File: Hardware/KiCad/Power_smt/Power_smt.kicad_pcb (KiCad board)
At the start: 2 copper layers, 38.1 x 25.4 mm, 11 parts

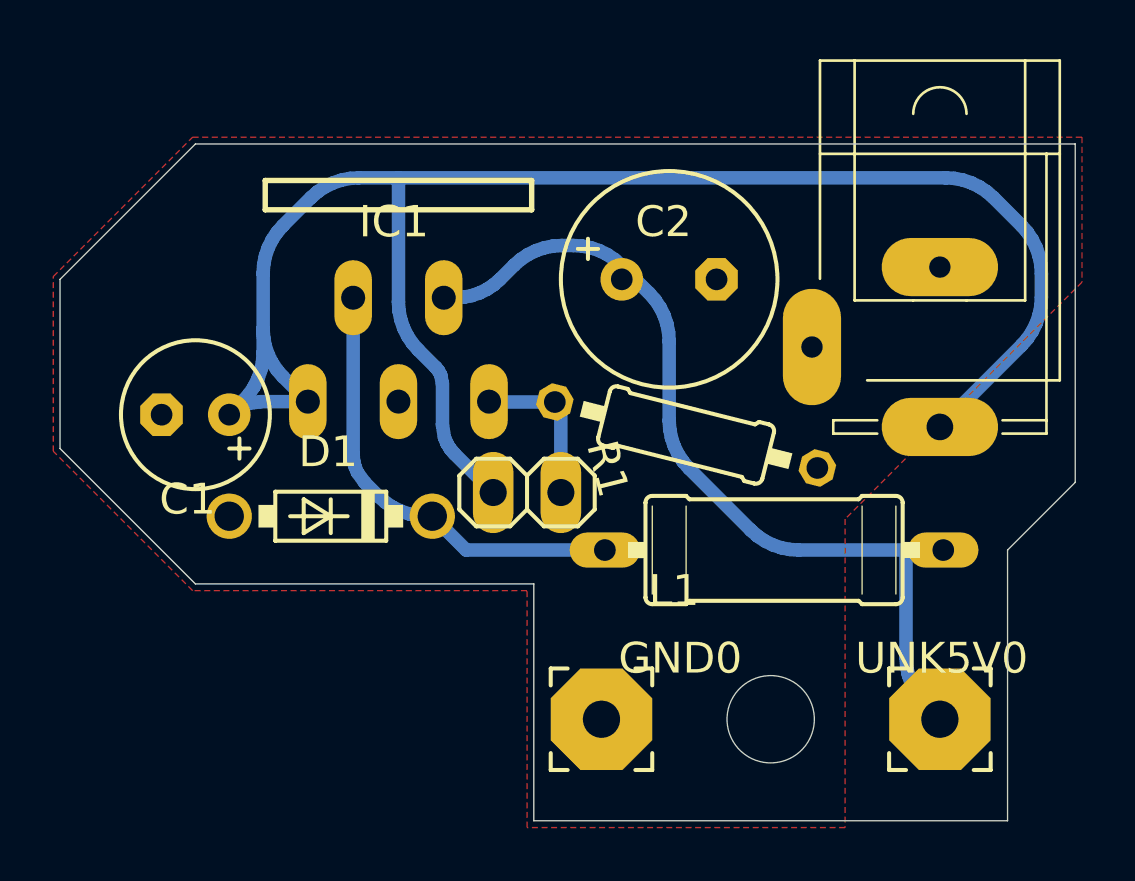
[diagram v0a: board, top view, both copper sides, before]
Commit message: power board kicad smt
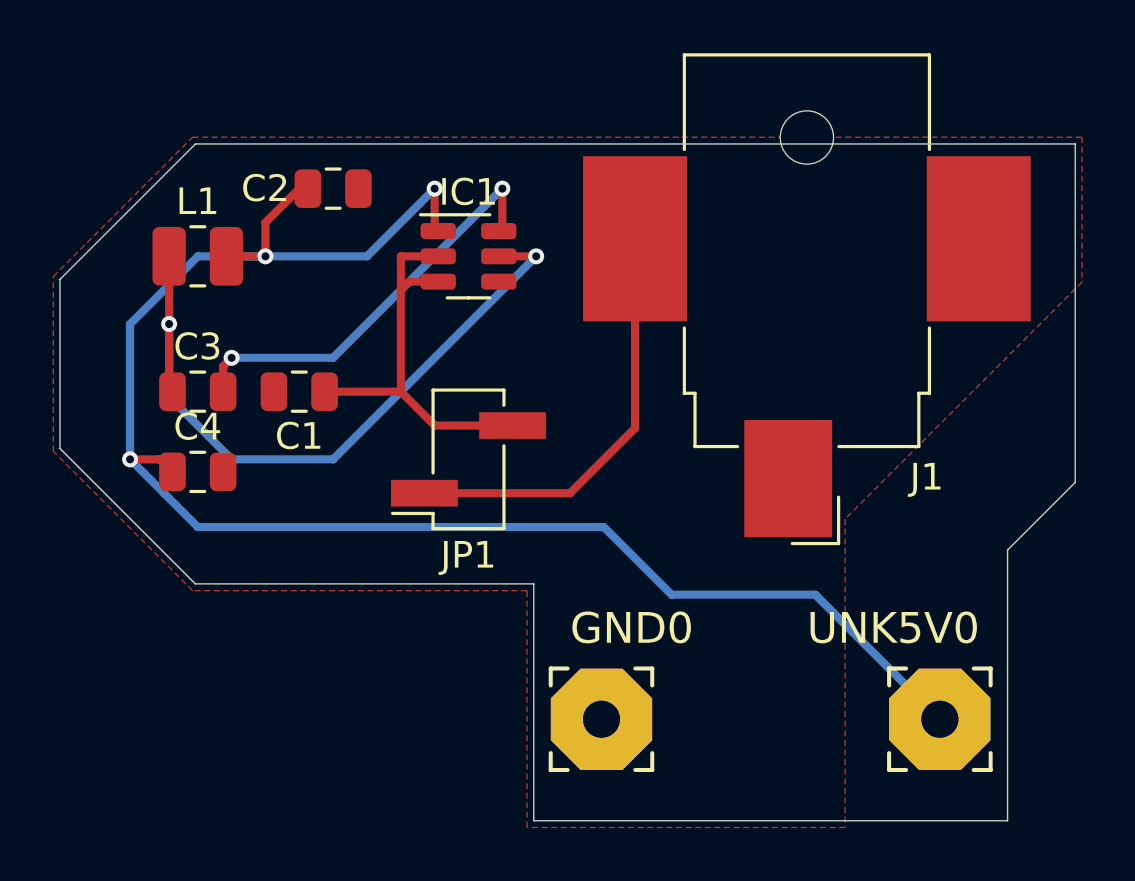
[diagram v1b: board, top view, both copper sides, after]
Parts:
- removed @HOLE0: , 
- removed D1: 1N5819-B, switched-lm2575:DO41-7.6
- removed R1: , switched-lm2575:0207_10
- added C3: 100nF, Capacitor_SMD:C_0805_2012Metric, F.Cu at (134.6, 101.6)
- added C4: 22uF, Capacitor_SMD:C_0805_2012Metric, F.Cu at (134.6, 104.6)
- C1: value 100uF -> 10uF; footprint switched-lm2575:E2,5-6 -> Capacitor_SMD:C_0805_2012Metric
- C2: value 330uF -> 22uF; footprint switched-lm2575:E3,5-8 -> Capacitor_SMD:C_0805_2012Metric
- GND0, UNK5V0: value (none) -> 3,81/1,4
- IC1: value (none) -> LM2596TV; footprint switched-lm2575:TO220-51 -> Package_TO_SOT_SMD:TSOT-23-6
- J1: value (none) -> JACK-PLUG0; footprint switched-lm2575:SPC4077 -> Connector_BarrelJack:BarrelJack_CUI_PJ-036AH-SMT_Horizontal
- JP1: value (none) -> PINHD-1X2; footprint switched-lm2575:1X02 -> Connector_PinHeader_2.54mm:PinHeader_1x02_P2.54mm_Vertical_SMD_Pin1Right
- L1: value 470uH -> 4.7uH; footprint switched-lm2575:SMCC12 -> Inductor_SMD:L_1008_2520Metric
- moved L1 24.3 mm to (134.6, 96.5)
- moved C2 13.1 mm to (139.7, 94.0)
- moved J1 5.07 mm to (157.5, 99.1), turned to 180 degrees
- moved C1 3.99 mm to (138.4, 101.6)
- moved IC1 3.95 mm to (144.8, 96.5)
- moved JP1 2.53 mm to (144.8, 104.1)
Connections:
- IC1 pad 1: VIN -> VCC
- IC1 pad 2: N$2 -> Net-(IC1-EN)
- IC1 pad 3: GND -> Net-(IC1-EN)
- IC1 pad 4: VCC -> GND
- IC1 pad 5: N$3 -> Net-(IC1-SW)
- J1 pad 2: (no net) -> unconnected-(J1-Pad2)
- J1 pad 3: VIN -> Net-(J1-Pad3)
- JP1 pad 1: N$3 -> Net-(J1-Pad3)
- JP1 pad 2: VIN -> Net-(IC1-EN)
- L1 pad 1: N$2 -> Net-(IC1-SW)
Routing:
- net VIN: track 65.4 -> 0.00 mm
- net VCC: track 33.9 -> 61.3 mm, vias 0 -> 3
- net Net-(IC1-SW): track 0.00 -> 27.2 mm, vias 0 -> 2
- net N$2: track 17.0 -> 0.00 mm
- net Net-(J1-Pad3): track 0.00 -> 16.0 mm
- net Net-(IC1-BST): track 0.00 -> 15.8 mm, vias 0 -> 2
- net Net-(IC1-EN): track 0.00 -> 15.6 mm
- net N$3: track 5.97 -> 0.00 mm
